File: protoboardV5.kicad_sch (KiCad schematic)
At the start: 17 parts, among them J1 J1, J2 J2, J3 J3, M1 M1, Q1 Q1, Q2 Q2, U1 U1

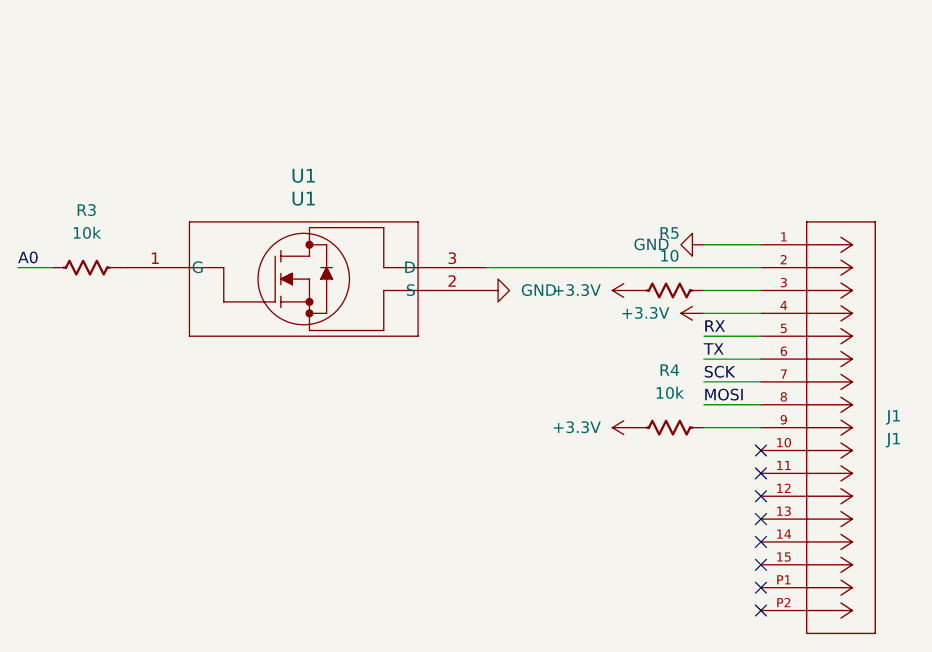
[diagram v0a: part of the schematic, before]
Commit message: Add files via upload
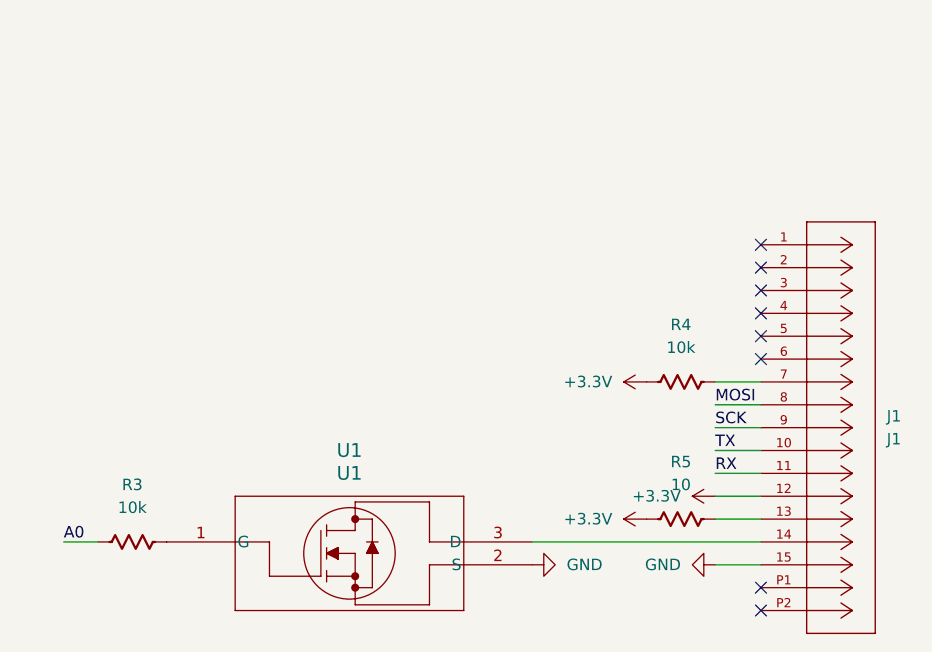
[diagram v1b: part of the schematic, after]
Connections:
- net +3.3V: now also J1.12; no longer J1.4
- net GND: now also J1.15; no longer J1.1
- net RX: now also J1.11; no longer J1.5
- net SCK: now also J1.9; no longer J1.7
- net TX: now also J1.10; no longer J1.6
- net at R4.2: now also J1.7; no longer J1.9
- net at J1.13: now also R5.2
- net at J1.14: now also U1.3 (D)
- net at J1.2: no longer U1.3 (D)
- net at J1.3: no longer R5.2
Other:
- moved on the sheet: R3, R4, R5, U1
